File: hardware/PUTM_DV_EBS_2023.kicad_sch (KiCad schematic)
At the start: 0 parts

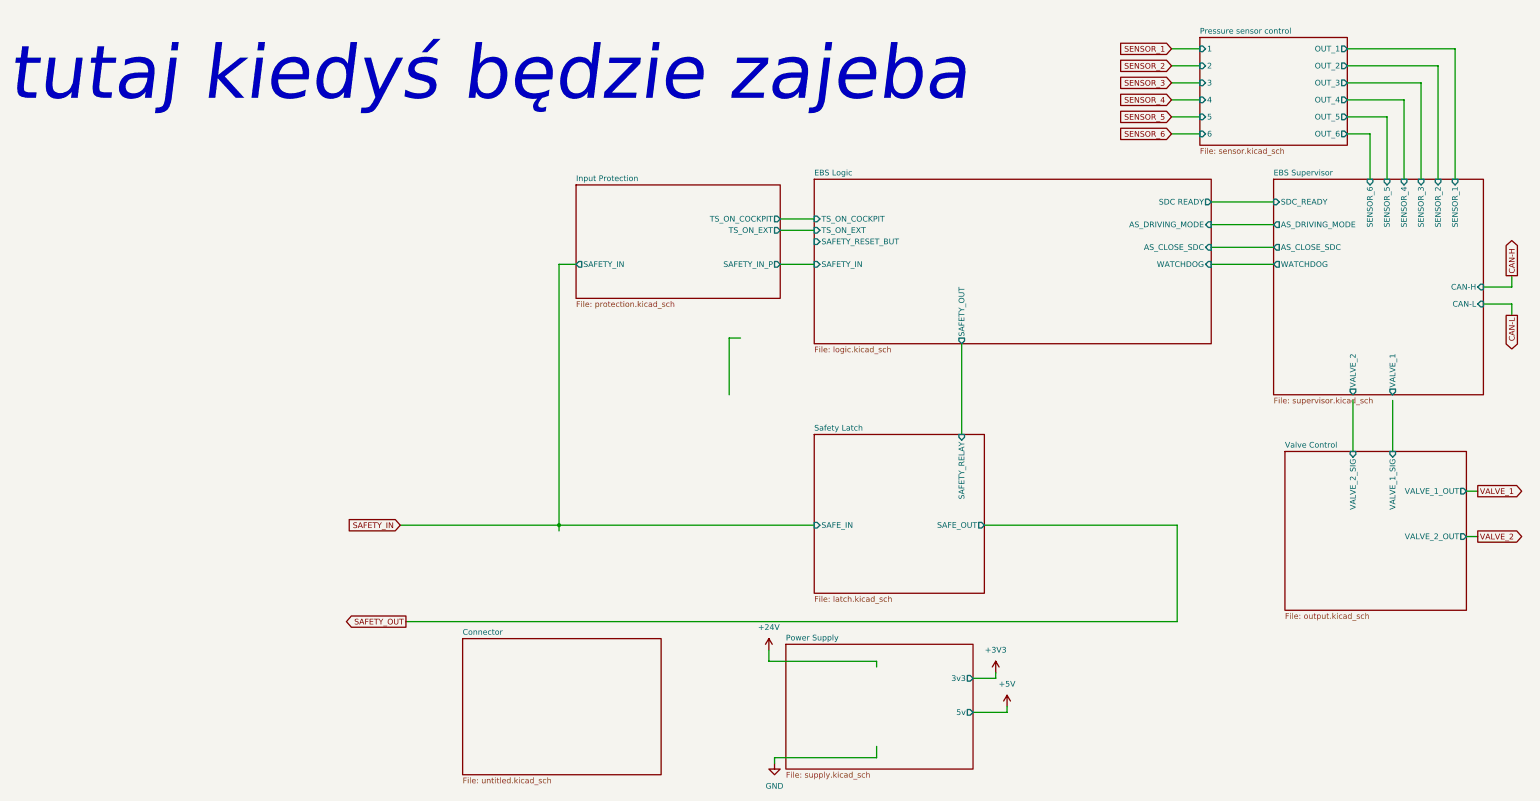
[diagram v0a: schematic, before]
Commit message: Fixed Logic
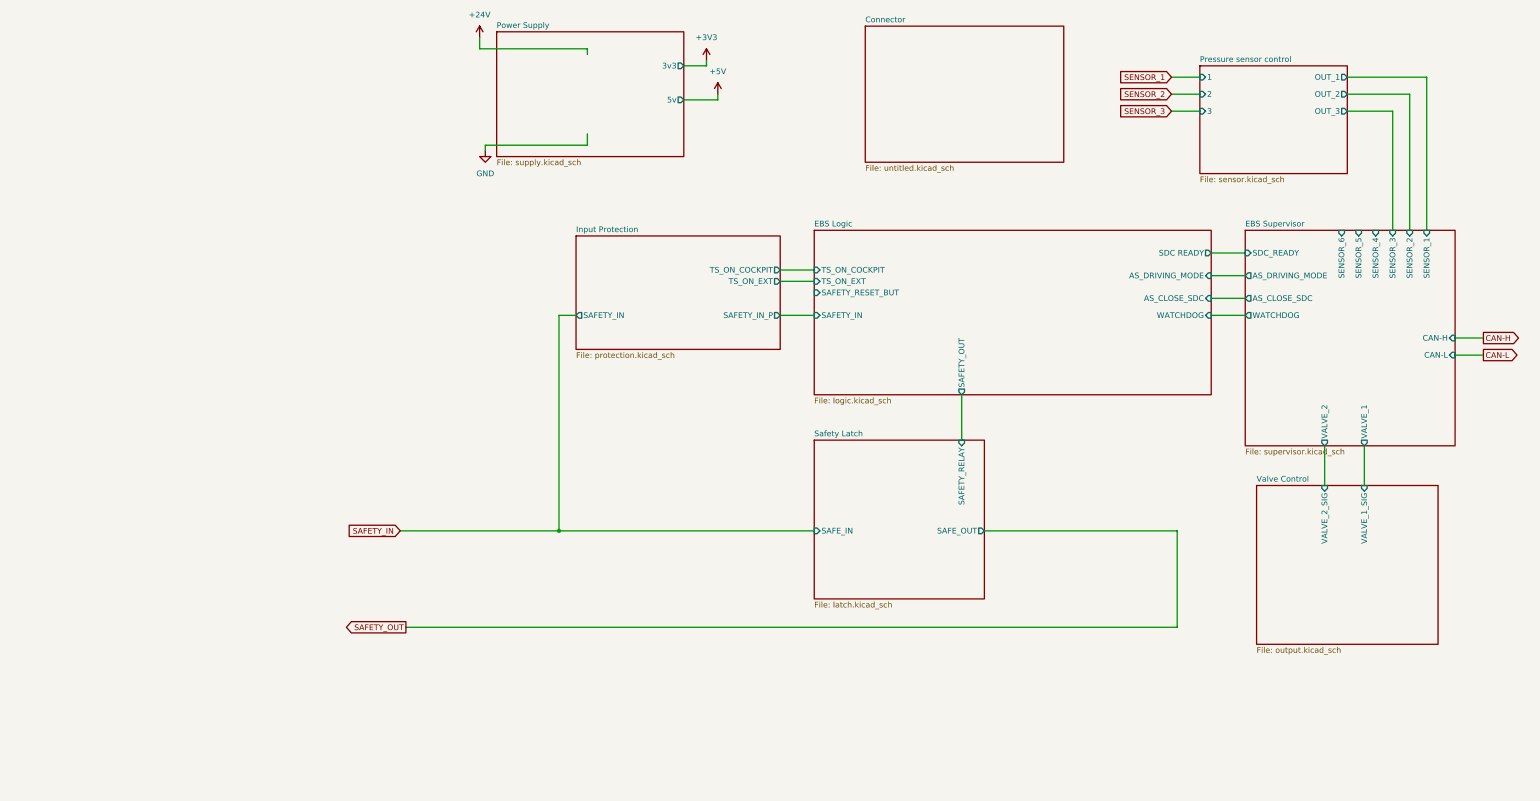
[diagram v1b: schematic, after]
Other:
- sheet Pressure sensor control ports: added none; removed 4, 5, 6, OUT_4, OUT_5, OUT_6
- sheet Valve Control ports: added none; removed VALVE_1_OUT, VALVE_2_OUT
- note removed: "tutaj kiedyś będzie zajeba"
